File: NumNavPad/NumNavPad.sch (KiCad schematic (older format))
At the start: 55 parts, among them U1 Elite-C

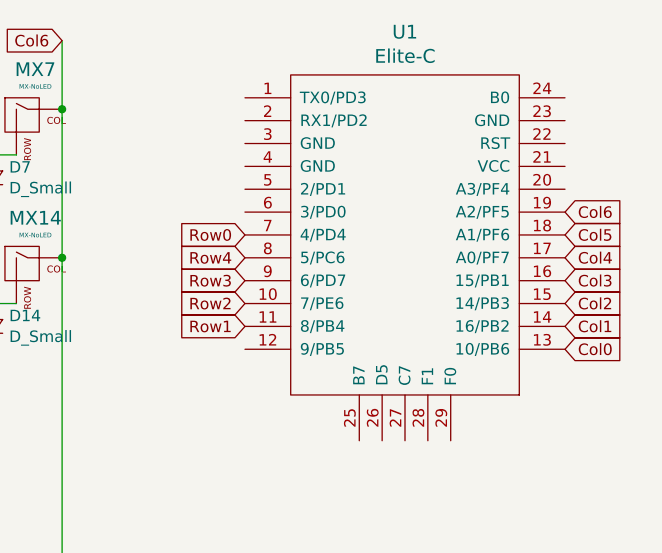
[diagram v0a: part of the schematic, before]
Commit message: Gerbers Added
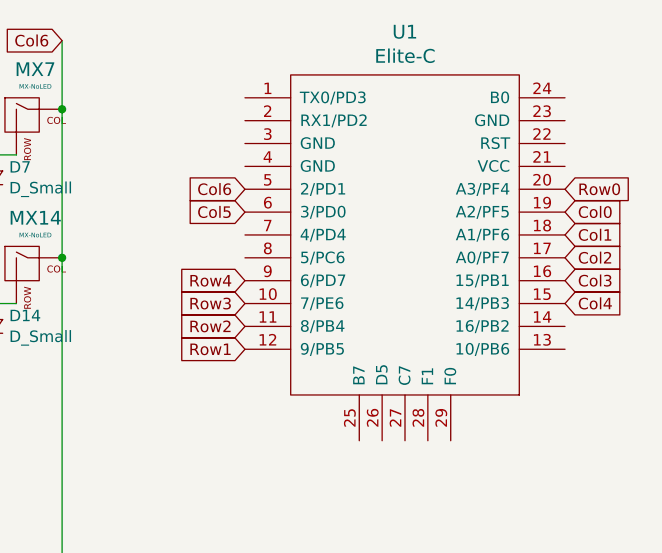
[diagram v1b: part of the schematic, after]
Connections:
- net Col0: now also U1.19 (A2/PF5); no longer U1.13 (10/PB6)
- net Col1: now also U1.18 (A1/PF6); no longer U1.14 (16/PB2)
- net Col2: now also U1.17 (A0/PF7); no longer U1.15 (14/PB3)
- net Col4: now also U1.15 (14/PB3); no longer U1.17 (A0/PF7)
- net Col5: now also U1.6 (3/PD0); no longer U1.18 (A1/PF6)
- net Col6: now also U1.5 (2/PD1); no longer U1.19 (A2/PF5)
- net Row0: now also U1.20 (A3/PF4); no longer U1.7 (4/PD4)
- net Row1: now also U1.12 (9/PB5); no longer U1.11 (8/PB4)
- net Row2: now also U1.11 (8/PB4); no longer U1.10 (7/PE6)
- net Row3: now also U1.10 (7/PE6); no longer U1.9 (6/PD7)
- net Row4: now also U1.9 (6/PD7); no longer U1.8 (5/PC6)
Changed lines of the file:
@@
 	1    0    0    -1
 $EndComp
-Text GLabel 5100 1850 0    50   Input ~ 0
+Text GLabel 6500 1650 2    50   Input ~ 0
 Row0
+Text GLabel 5100 2350 0    50   Input ~ 0
+Row1
 Text GLabel 5100 2250 0    50   Input ~ 0
-Row1
+Row2
 Text GLabel 5100 2150 0    50   Input ~ 0
-Row2
+Row3
 Text GLabel 5100 2050 0    50   Input ~ 0
-Row3
-Text GLabel 5100 1950 0    50   Input ~ 0
 Row4
-Text GLabel 6500 2350 2    50   Input ~ 0
+Text GLabel 6500 1750 2    50   Input ~ 0
 Col0
-Text GLabel 6500 2250 2    50   Input ~ 0
+Text GLabel 6500 1850 2    50   Input ~ 0
 Col1
-Text GLabel 6500 2150 2    50   Input ~ 0
+Text GLabel 6500 1950 2    50   Input ~ 0
 Col2
 Text GLabel 6500 2050 2    50   Input ~ 0
 Col3
-Text GLabel 6500 1950 2    50   Input ~ 0
+Text GLabel 6500 2150 2    50   Input ~ 0
 Col4
-Text GLabel 6500 1850 2    50   Input ~ 0
+Text GLabel 5100 1750 0    50   Input ~ 0
 Col5
-Text GLabel 6500 1750 2    50   Input ~ 0
+Text GLabel 5100 1650 0    50   Input ~ 0
 Col6
 $EndSCHEMATC
